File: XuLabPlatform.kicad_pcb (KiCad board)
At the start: 2 copper layers, 83 x 116.5 mm, 73 parts, among them J1 SWD Connector, J10 Servo7, J11 Servo8, J12 Thruster SGN, J13 USB_B_Micro, J14 CAN, J15 I2C, J16 UART, J2 Conn_01x04, J3 1986660-2, J4 Servo1, J5 Servo2, J6 Servo3, J7 Servo4, J8 Servo5, J9 Servo6, Q2 PMOS, SW1 SW_Push, SW2 SW_SPDT, SW3 SW_SPDT, U1 STM32F446RCTx, U2 ISM330DHCX, U3 MMC5983MA, U4 AP63203WU, U5 TVS0500DRV, U6 TLV1117LV33, Y1 25 MHz

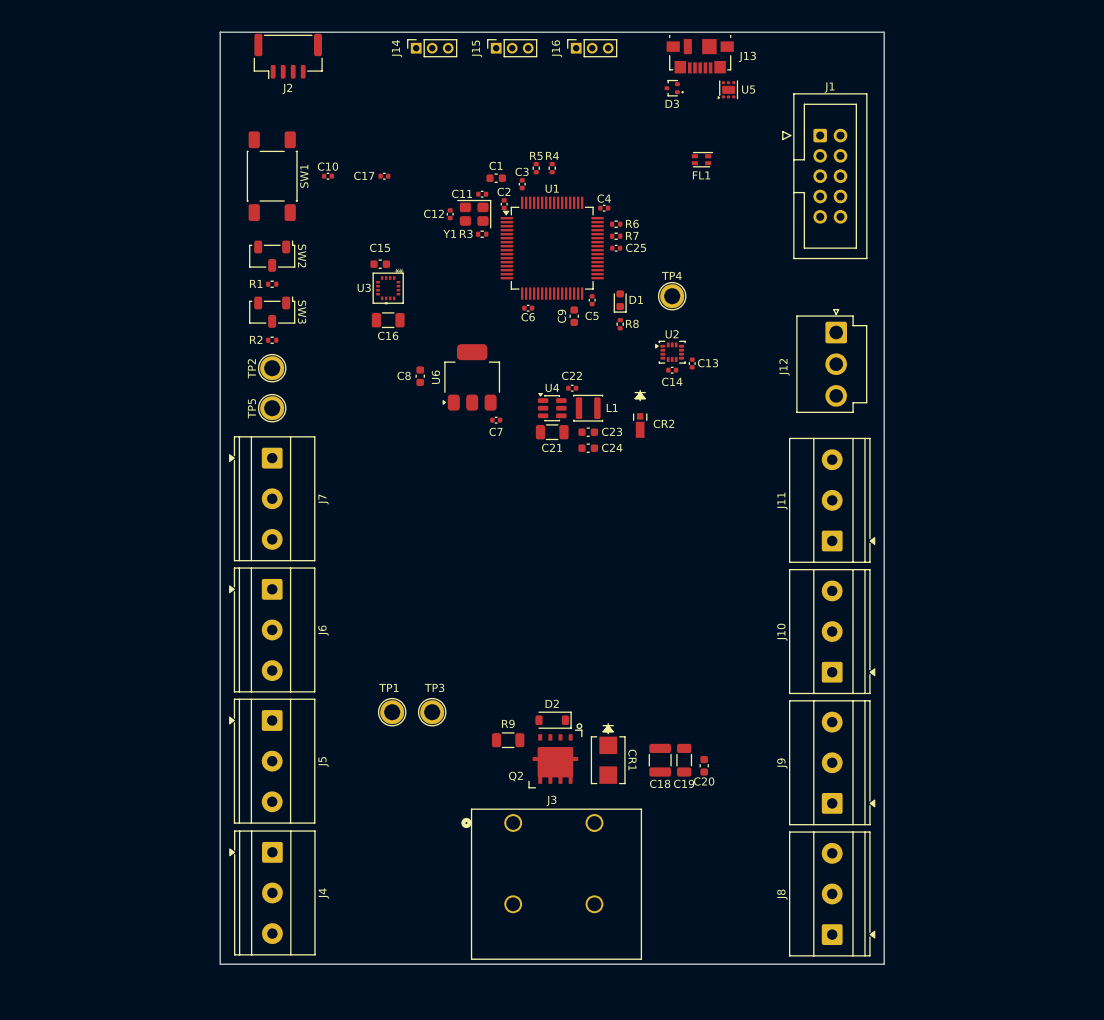
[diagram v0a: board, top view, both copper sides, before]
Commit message: Update layout
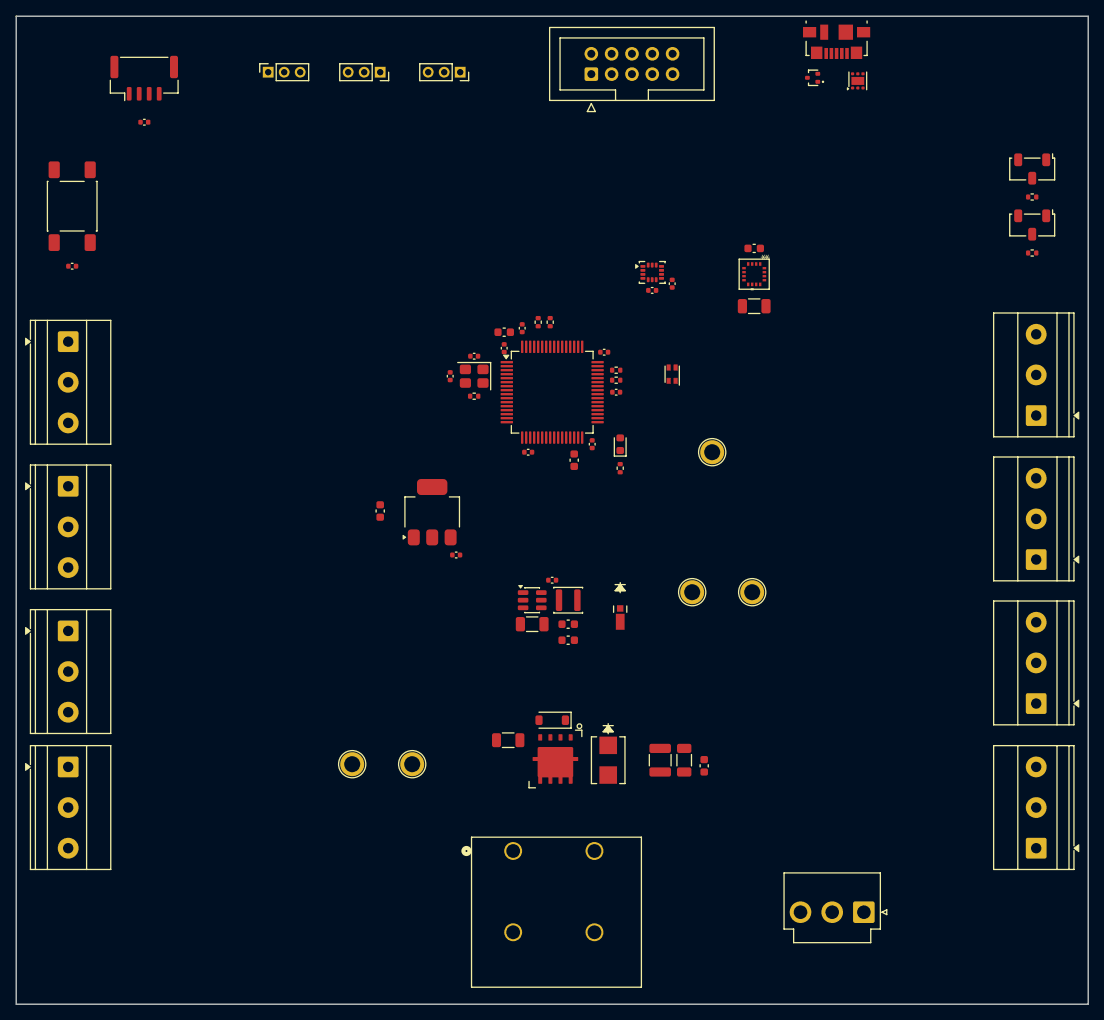
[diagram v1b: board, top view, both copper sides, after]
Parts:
- moved R1 95.6 mm to (210.0, 55.6)
- moved R2 95.6 mm to (210.0, 62.6)
- moved SW2 95.6 mm to (210.0, 52.1)
- moved SW3 95.6 mm to (210.0, 59.1)
- moved J12 72.5 mm to (189.0, 145.0), turned to 180 degrees
- moved TP5 64.3 mm to (175.0, 105.0), turned to 180 degrees
- moved TP2 59.5 mm to (167.5, 105.0), turned to -90 degrees
- moved C15 46.8 mm to (175.2, 62.0)
- moved C16 45.8 mm to (175.2, 69.2)
- moved U3 45.8 mm to (175.2, 65.2)
- moved C10 33.9 mm to (90.0, 64.2)
- moved C17 30.8 mm to (99.0, 46.2), turned to 0 degrees
- moved J11 29.9 mm to (210.5, 82.9)
- moved J1 29.6 mm to (154.9, 40.2), turned to 90 degrees
- moved J7 29.4 mm to (89.5, 73.7)
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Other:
- board size 83 x 116.5 mm -> 134 x 123.5 mm
